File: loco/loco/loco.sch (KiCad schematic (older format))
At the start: 3 parts, among them U1 STM32F030F4Px, U2 A4953_LJ

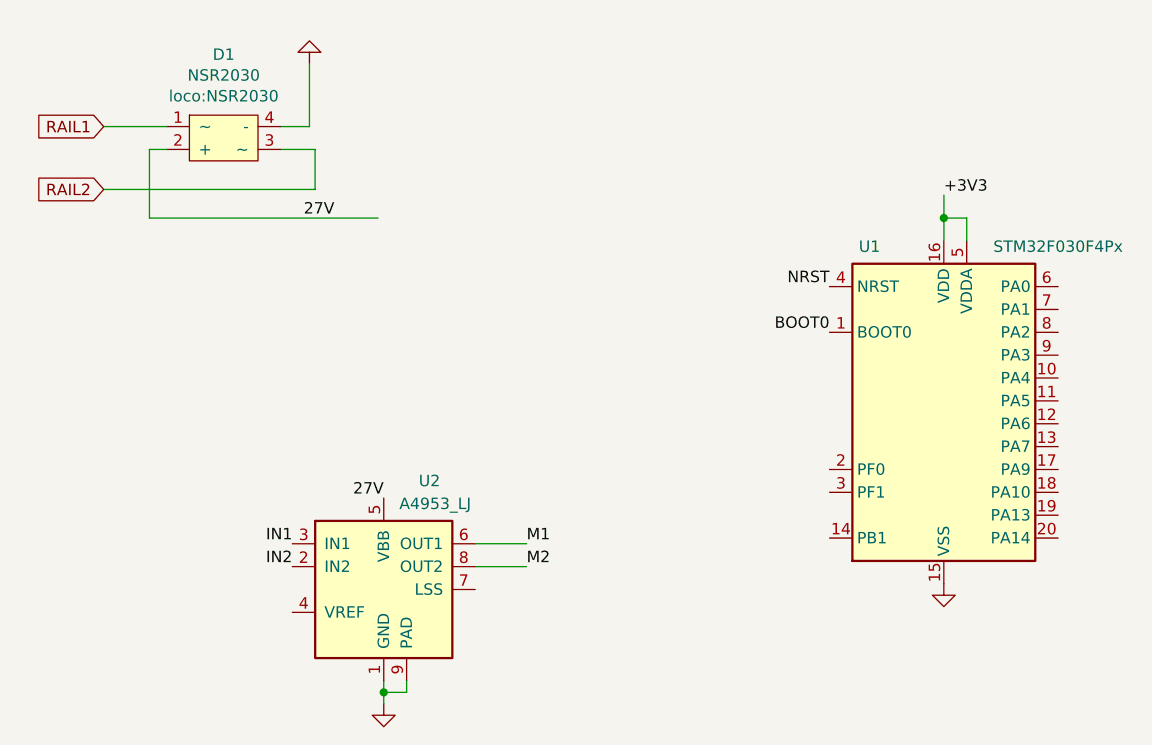
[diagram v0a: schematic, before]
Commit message: Up
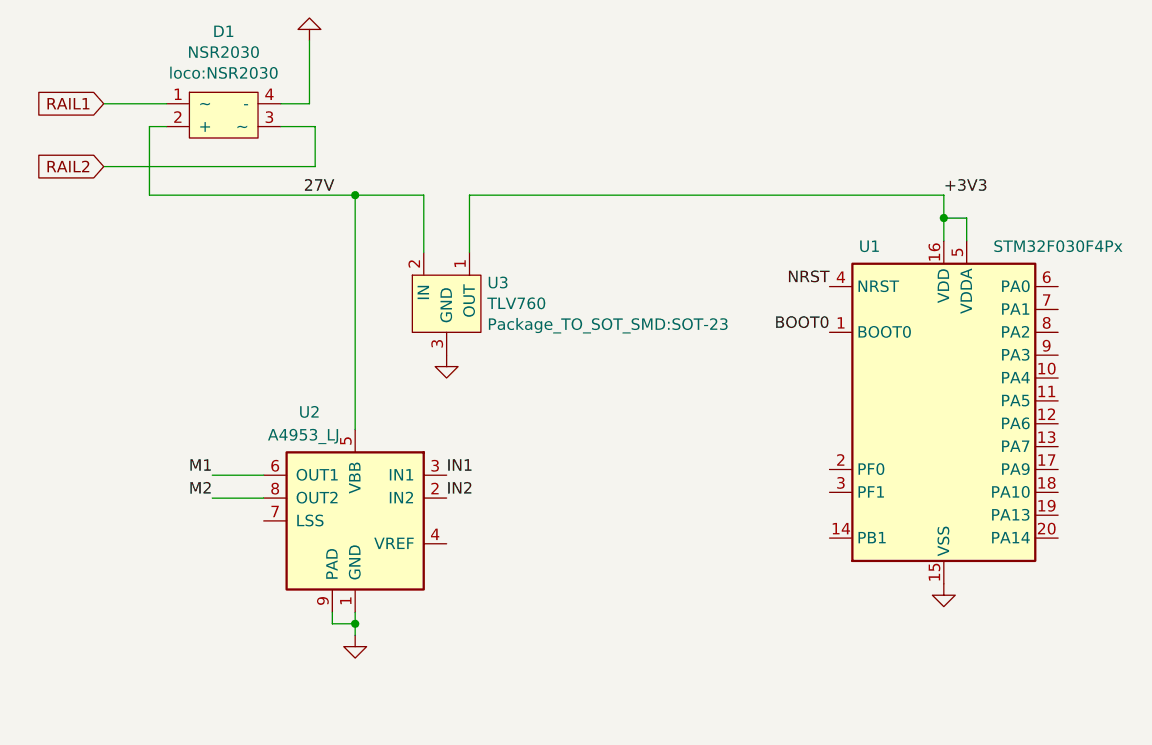
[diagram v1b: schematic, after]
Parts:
- added U3: TLV760, Package_TO_SOT_SMD:SOT-23, symbol loco:TLV760
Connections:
- wire segments 19 -> 24
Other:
- moved on the sheet: D1, U2
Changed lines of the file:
@@
 L loco:NSR2030 D1
 U 1 1 5E65250C
-P 2500 2350
-F 0 "D1" H 2500 2715 50  0000 C CNN
-F 1 "NSR2030" H 2500 2624 50  0000 C CNN
-F 2 "loco:NSR2030" H 2500 2533 50  0000 C CNN
-F 3 "" H 2500 2350 50  0001 C CNN
-	1    2500 2350
+P 2500 2250
+F 0 "D1" H 2500 2615 50  0000 C CNN
+F 1 "NSR2030" H 2500 2524 50  0000 C CNN
+F 2 "loco:NSR2030" H 2500 2433 50  0000 C CNN
+F 3 "" H 2500 2250 50  0001 C CNN
+	1    2500 2250
 	1    0    0    -1
 $EndComp
 Wire Wire Line
-	2750 2400 2900 2400
+	2750 2300 2900 2300
 Wire Wire Line
-	2900 2400 2900 2575
+	2900 2300 2900 2475
 Wire Wire Line
-	2900 2575 1975 2575
+	2900 2475 1975 2475
 Wire Wire Line
-	2250 2300 1975 2300
-Text GLabel 1975 2300 0    50   Input ~ 0
+	2250 2200 1975 2200
+Text GLabel 1975 2200 0    50   Input ~ 0
 RAIL1
-Text GLabel 1975 2575 0    50   Input ~ 0
+Text GLabel 1975 2475 0    50   Input ~ 0
 RAIL2
 $Comp
 L power:GND #PWR0102
 U 1 1 5E652E8A
-P 2875 2025
-F 0 "#PWR0102" H 2875 1775 50  0001 C CNN
-F 1 "GND" H 2880 1852 50  0001 C CNN
-F 2 "" H 2875 2025 50  0001 C CNN
-F 3 "" H 2875 2025 50  0001 C CNN
-	1    2875 2025
+P 2875 1925
+F 0 "#PWR0102" H 2875 1675 50  0001 C CNN
+F 1 "GND" H 2880 1752 50  0001 C CNN
+F 2 "" H 2875 1925 50  0001 C CNN
+F 3 "" H 2875 1925 50  0001 C CNN
+	1    2875 1925
 	-1   0    0    1
 $EndComp
 Wire Wire Line
-	2875 2025 2875 2300
+	2875 1925 2875 2200
 Wire Wire Line
-	2875 2300 2750 2300
+	2875 2200 2750 2200
 Wire Wire Line
-	2250 2400 2175 2400
+	2250 2300 2175 2300
 Wire Wire Line
-	2175 2400 2175 2700
+	2175 2300 2175 2600
 Wire Wire Line
-	2175 2700 3175 2700
+	2175 2600 3075 2600
 $Comp
 L Driver_Motor:A4953_LJ U2
 U 1 1 5E653C2B
-P 3200 4325
-F 0 "U2" H 3400 4800 50  0000 C CNN
-F 1 "A4953_LJ" H 3425 4700 50  0000 C CNN
-F 2 "Package_SO:SOIC-8-1EP_3.9x4.9mm_P1.27mm_EP2.41x3.3mm" H 3200 3775 50  0001 C CNN
-F 3 "www.allegromicro.com/~/media/Files/Datasheets/A4952-3-Datasheet.ashx?la=en" H 2900 4675 50  0001 C CNN
-	1    3200 4325
-	1    0    0    -1
+P 3075 4025
+F 0 "U2" H 3275 4500 50  0000 C CNN
+F 1 "A4953_LJ" H 3300 4400 50  0000 C CNN
+F 2 "Package_SO:SOIC-8-1EP_3.9x4.9mm_P1.27mm_EP2.41x3.3mm" H 3075 3475 50  0001 C CNN
+F 3 "www.allegromicro.com/~/media/Files/Datasheets/A4952-3-Datasheet.ashx?la=en" H 2775 4375 50  0001 C CNN
+	1    3075 4025
+	-1   0    0    -1
 $EndComp
-Text Label 2850 2700 0    50   ~ 0
+Text Label 2850 2600 0    50   ~ 0
 27V
 Text Label 5150 3000 2    50   ~ 0
@@
 +3V3
 $Comp
-L power:GND #PWR?
+L power:GND #PWR0103
 U 1 1 5E657AD9
-P 3200 4825
-F 0 "#PWR?" H 3200 4575 50  0001 C CNN
-F 1 "GND" H 3205 4652 50  0001 C CNN
-F 2 "" H 3200 4825 50  0001 C CNN
-F 3 "" H 3200 4825 50  0001 C CNN
-	1    3200 4825
+P 3075 4525
+F 0 "#PWR0103" H 3075 4275 50  0001 C CNN
+F 1 "GND" H 3080 4352 50  0001 C CNN
+F 2 "" H 3075 4525 50  0001 C CNN
+F 3 "" H 3075 4525 50  0001 C CNN
+	1    3075 4525
+	-1   0    0    -1
+$EndComp
+Wire Wire Line
+	3075 4425 3075 4475
+Wire Wire Line
+	2975 4425 2975 4475
+Wire Wire Line
+	2975 4475 3075 4475
+Connection ~ 3075 4475
+Wire Wire Line
+	3075 4475 3075 4525
+Wire Wire Line
+	2675 3825 2450 3825
+Wire Wire Line
+	2675 3925 2450 3925
+Text Label 2450 3825 2    50   ~ 0
+M1
+Text Label 2450 3925 2    50   ~ 0
+M2
+Text Label 3475 3825 0    50   ~ 0
+IN1
+Text Label 3475 3925 0    50   ~ 0
+IN2
+$Comp
+L loco:TLV760 U3
+U 1 1 5E653E6E
+P 3475 3100
+F 0 "U3" H 3653 3216 50  0000 L CNN
+F 1 "TLV760" H 3653 3125 50  0000 L CNN
+F 2 "Package_TO_SOT_SMD:SOT-23" H 3653 3034 50  0000 L CNN
+F 3 "" H 3475 3200 50  0001 C CNN
+	1    3475 3100
+	1    0    0    -1
+$EndComp
+$Comp
+L power:GND #PWR0104
+U 1 1 5E654599
+P 3475 3300
+F 0 "#PWR0104" H 3475 3050 50  0001 C CNN
+F 1 "GND" H 3480 3127 50  0001 C CNN
+F 2 "" H 3475 3300 50  0001 C CNN
+F 3 "" H 3475 3300 50  0001 C CNN
+	1    3475 3300
 	1    0    0    -1
 $EndComp
 Wire Wire Line
-	3200 4725 3200 4775
+	3375 2600 3375 2850
 Wire Wire Line
-	3300 4725 3300 4775
+	3575 2850 3575 2600
 Wire Wire Line
-	3300 4775 3200 4775
-Connection ~ 3200 4775
+	3575 2600 5650 2600
 Wire Wire Line
-	3200 4775 3200 4825
+	3075 3625 3075 2600
+Connection ~ 3075 2600
 Wire Wire Line
-	3600 4125 3825 4125
-Wire Wire Line
-	3600 4225 3825 4225
-Text Label 3825 4125 0    50   ~ 0
-M1
-Text Label 3825 4225 0    50   ~ 0
-M2
-Text Label 2800 4125 2    50   ~ 0
-IN1
-Text Label 2800 4225 2    50   ~ 0
-IN2
-Text Label 3200 3925 2    50   ~ 0
-27V
+	3075 2600 3375 2600
 $EndSCHEMATC
